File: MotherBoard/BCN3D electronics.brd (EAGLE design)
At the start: 80 x 140 mm, 139 parts, among them IC2 FT232RL, IC3 LMV324MZ, K1 G5L, Q1 MOSFET-N, Q2 MOSFET-N, Q3 MOSFET-N, Q4 BC817, Q5 BC817, Q9 BC817, X0 FFC_15V_90G_1MM, X1 FFC_15V_90G_1MM, Y0 FFC_15V_90G_1MM

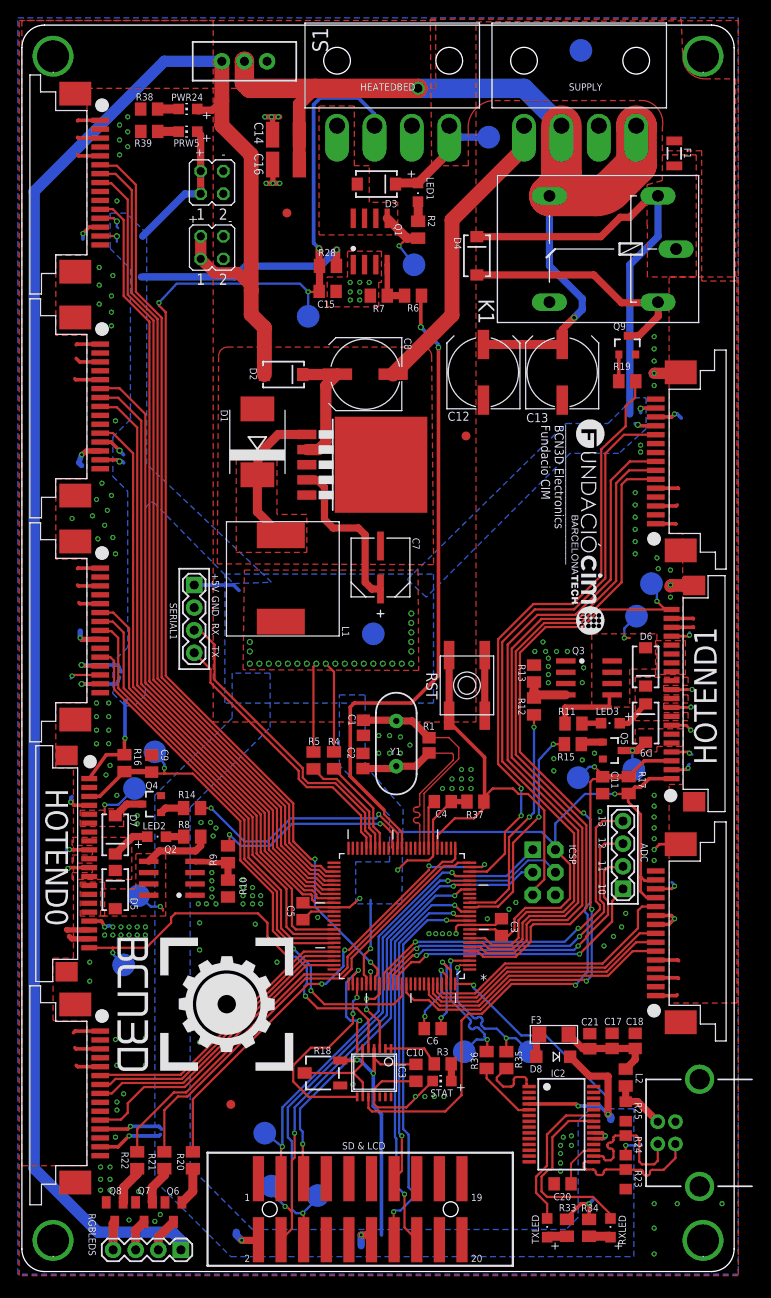
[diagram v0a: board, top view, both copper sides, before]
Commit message: BCN3D Electronics REV.E tested and manufactured
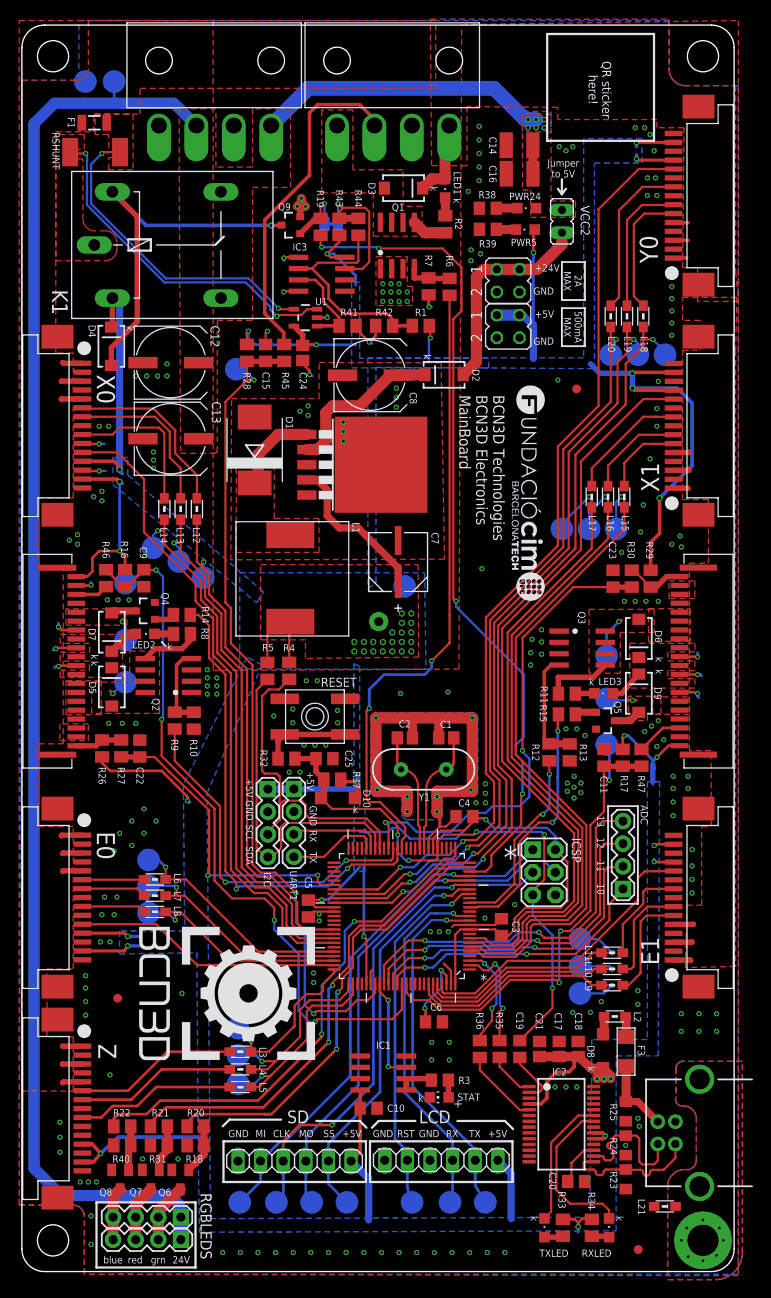
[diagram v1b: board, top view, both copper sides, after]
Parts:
- removed HTST1: HTST_20V_SMD_POL, MarcEagleParts:HTST-110-01-XX-DV
- removed JP1: +5V, jumper:JP2Q
- removed JP2: +24V, jumper:JP2Q
- removed PRW5: Red, adafruit:CHIP-LED0805
- removed RST: SPST_TACT-EVQQ2, adafruit:EVQ-Q2
- removed S1: (no value), SparkFun-Electromechanical:SWITCH-SPDT
- removed SERIAL1: (no value), SparkFun-Connectors:1X04
- removed TP14, TP18, TP6: TPB2,54, testpad:B2,54
- removed U$2, U$3, U$4: SANGUINOLOLU_PLATED-SCREW, SAV MK-I:SANGUINOLOLU_PLATEDSCREW
- added +24V, +5V: (no value), jumper:JP2Q
- added C19: 100n, rcl:C0805
- added C22, C23: 0.1u, rcl:C0805
- added C24: 100n, adafruit:C0805
- added C25: 10n, rcl:C0805
- added D10: MBR0520LT, diode:SOD123
- added I2C, LEDS1, UART1: (no value), SparkFun-Connectors:1X04
- added IC1: LM358D, linear:SO08
- added L10, L11, L12, L13, L14, L15, L16, L17, L18, L19, L20, L21, L3, L4, L5, L6, L7, L8, L9: (no value), EagleLibrary_Wuerth_Elektronik_eiSos_V6_20140807:0805
- added LCD, SD: (no value), pinhead:1X06
- added PWR5: Blue, led:CHIPLED_0805
- added R26, R29: 4.7K, rcl:M0805
- added R27, R30, R43, R45, R46, R47: 1K, rcl:M0805
- added R31, R40, R42: 10K, rcl:M0805
- added R32: 330, adafruit:M0805
- added R41: 20K, rcl:M0805
- added R44: 100K, rcl:M0805
- added RESET: SPST, adafruit:EVQ-Q2
- added RSHUNT: 10m, SparkFun-Resistors:R2512
- added SH1: SHORTT5, shorts:SHORT_TOP-50
- added SJ1: (no value), jumper:SJ
- added TP19, TP20, TP21, TP22, TP23, TP24, TP25, TP26, TP27, TP28, TP29, TP30, TP31, TP32, TP33, TP34, TP35, TP36, TP37, TP38: TPB2,54, testpad:B2,54
- added U1: INA169, SparkFun-AnalogIC:SOT23-5
- added VCC2: (no value), jumper:JP1
- C11, C15, C9: value 0.1u -> 10u
- HOTEND0, HOTEND1: value FFC_20V_90G_1MM" -> FFC_20V_90G_1MM3; device MarcEagleParts:SAMTEC_ZF1-T-WT -> MarcEagleParts:FCI_20WAY_1MM_3ST
- IC3: value LMV324MZ -> LM311D; device linear:TSSOP14 -> linear:SO08
- ICSP: value (none) -> AVR_SPI_PRG_6NS
- L2: value 1800367 Ferrite Bead -> (none); device rcl:M0805 -> EagleLibrary_Wuerth_Elektronik_eiSos_V6_20140807:0805
- LED1, LED2, LED3: value (none) -> Blue
- LM2595: device linear:TO263-5 -> MarcEagleParts:TO263-5
- PWR24: value Red -> Blue; device adafruit:CHIP-LED0805 -> led:CHIPLED_0805
- Q1, Q2, Q3: value MOSFET-N -> MOSFET-NSOIC8
- Q4, Q5, Q9: value BC817 -> MMBT2222A
- R1: value 1M -> 10K; device resistor:R0805 -> rcl:M0805
- R18: device pot:3223J -> rcl:M0805
- R4, R5: value 10K -> 4.7k
- U$1: value SANGUINOLOLU_PLATED-SCREW -> (none); device SAV MK-I:SANGUINOLOLU_PLATEDSCREW -> MarcEagleParts:BCN3D_QR
- moved Z 114.0 mm to (4.00, 18.3)
- moved U$1 112.6 mm to (60.4, 100.7), flipped to the bottom, turned to 270 degrees
- moved FID1 93.4 mm to (69.2, 2.48)
- moved IC3 89.9 mm to (33.7, 112.0), turned to 270 degrees
- moved TP13 83.4 mm to (24.1, 101.3), turned to 0 degrees
- moved TP5 73.1 mm to (48.1, 7.77), turned to 90 degrees
- moved Y0 71.3 mm to (76.0, 120.8), turned to 90 degrees
- moved F1 65.2 mm to (8.13, 129.0), turned to 180 degrees
- moved TP1 55.8 mm to (7.12, 133.7), turned to 0 degrees
- moved SUPPLY 47.2 mm to (21.9, 132.4)
- moved R1 47.1 mm to (44.8, 106.2), turned to 180 degrees
- moved K1 46.3 mm to (17.7, 115.3), turned to 0 degrees
- moved C13 44.6 mm to (16.7, 93.5), turned to 0 degrees
- moved TP2 42.5 mm to (10.4, 133.7), turned to 0 degrees
- moved D4 42.3 mm to (10.1, 103.9)
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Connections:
- removed net ATLVL0: HOTEND0.20, IC3.5, TP4.TP
- removed net ATLVL1: HOTEND1.20, IC3.10, TP5.TP
- removed net H0-STOP: ATMEGA2560.77, IC3.7
- removed net H1-STOP: ATMEGA2560.78, IC3.8
- removed net N$108: C12.+, C13.+, C14.1, C16.1, K1.S, S1.2, SUPPLY.1, SUPPLY.3
- removed net N$110: IC3.6, IC3.9, R18.2
- removed net N$111: HTST1.8
- removed net N$112: HTST1.9
- removed net N$115: HTST1.10
- removed net N$116: HTST1.16
- removed net N$117: HTST1.17
- removed net N$118: HTST1.18
- removed net N$119: HTST1.19
- removed net N$120: HTST1.20
- removed net N$121: S1.1
- removed net N$124: ATMEGA2560.18
- removed net N$146: ATMEGA2560.41
- removed net N$25: Q9.1, R19.1
- removed net RX0: ATMEGA2560.2, R35.1, TP13.TP
- removed net TX0: ATMEGA2560.3, R36.1, TP14.TP
- removed net VBUSAF: C17.1, C18.1, C21.1, F3.2, L2.1
- new net 24VINA: K1.P, RSHUNT.1, U1.3
- new net BED_THERM_CON: HEATEDBED.3, R45.1
- new net EARTH: L21.2, U$6.S1, U$6.S2
- new net GUARD: C1.2, C2.2, SH1.2
- new net HOTEND0_THERM_CON: HOTEND0.3, R46.1
- new net HOTEND1_THERM_CON: HOTEND1.3, R47.1
- new net INA_OUT: IC3.3, R41.2, U1.1
- new net N$1: C19.1, IC2.2
- new net N$34: L13.1, X0.7
- new net N$35: L14.1, X0.9
- new net N$36: L18.1, Y0.6
- new net N$37: L19.1, Y0.7
- new net N$39: L20.1, Y0.9
- new net N$4: ATMEGA2560.14
- new net N$40: L15.1, X1.6
- new net N$41: L16.1, X1.7
- new net N$42: L17.1, X1.9
- new net N$43: E0.6, L6.2
- new net N$44: E0.7, L7.2
- new net N$45: E0.9, L8.2
- new net N$47: ATMEGA2560.55
- new net N$48: F3.2, L2.1
- new net N$49: IC3.2, R1.2, R42.1, R44.1
- new net N$5: L12.1, X0.6
- new net N$54: L3.1, Z.6
- new net N$55: L4.1, Z.7
- new net N$56: L5.1, Z.9
- new net N$57: E1.9, L11.1
- new net N$58: E1.7, L10.1
- new net N$59: E1.6, L9.1
- new net RELAYINA: IC3.7, Q9.1, R19.1, R43.2, R44.2, SJ1.1, SJ1.2
- new net SUPPLY: C12.+, C13.+, C14.1, C16.1, K1.S, LEDS1.1, PWR24.A, RGBLEDS.1, SUPPLY.1, SUPPLY.3, TP2.TP, VCC2.1
- new net UART_N: ATMEGA2560.3, R36.1
- new net UART_P: ATMEGA2560.2, R35.1
- new net Z0-ENDSTOP: HOTEND0.20, R26.1, R27.1
- new net Z0-STOP: ATMEGA2560.56, C22.1, R27.2
- new net Z1-ENDSTOP: HOTEND1.20, R29.1, R30.1
- new net Z1-STOP: ATMEGA2560.41, C23.1, R30.2
- net !RESET: now also C19.2, C25.1, D10.A, R32.1; no longer RST.A, RST.A'
- net +24V: now also Y0.GND@2; no longer HOTEND1.GND1, TP2.TP, Z.GND@1
- net +5V: now also +24V.1, +24V.3, C17.1, C18.1, C21.1, C24.1, D10.C, I2C.1, IC1.8, IC3.8, LCD.1, PWR5.A, R1.1, R26.2, R29.2, R43.1, SD.6, U1.5, UART1.1; no longer HTST1.1, HTST1.11, IC3.4, JP1.1, JP1.3, PRW5.A, R18.3, SERIAL1.1
- net 24VBF: now also RSHUNT.2, U1.4; no longer K1.P
- net BED_THERM: now also R45.2, TP13.TP; no longer HEATEDBED.3, TP18.TP
- net E0-!EN: now also L7.1, TP34.TP; no longer E0.7
- net E0-DIR: now also ATMEGA2560.73, L8.1, TP33.TP; no longer ATMEGA2560.71, E0.6
- net E0-STEP: now also ATMEGA2560.71, L6.1, TP35.TP; no longer ATMEGA2560.73, E0.8
- net E1-!EN: now also L10.2, TP31.TP; no longer E1.7
- net E1-DIR: now also ATMEGA2560.96, L11.2, TP32.TP; no longer ATMEGA2560.94, E1.6
- net E1-STEP: now also ATMEGA2560.94, L9.2, TP30.TP; no longer ATMEGA2560.96, E1.8
- net GND: now also +24V.2, +24V.4, +5V.2, +5V.4, C22.2, C23.2, C24.2, C25.2, E0.8, E1.8, HOTEND1.GND1, I2C.2, IC1.4, IC3.1, IC3.4, L21.1, LCD.4, LCD.6, R18.2, R31.2, R40.2, R41.1, R42.2, RESET.A, RESET.A', SD.1, SH1.1, U1.2, UART1.2, X0.8, X1.8, Y0.8, Z.8, Z.GND@1; no longer C1.2, C2.2, E0.9, E1.9, HTST1.12, HTST1.2, IC3.11, JP1.2, JP1.4, JP2.2, JP2.4, R18.1, RST.B, RST.B', SERIAL1.2, U$1.GND, U$2.GND, U$3.GND, U$4.GND, U$6.S1, U$6.S2, X0.9, X1.9, Y0.9, Y0.GND@2, Z.9
- net HOTBED: no longer TP6.TP
- net HOTEND0_THERM: now also R46.2; no longer HOTEND0.3
- net HOTEND1_THERM: now also R47.2; no longer HOTEND1.3
- net LCDRESET: now also ATMEGA2560.18, LCD.5, TP4.TP; no longer ATMEGA2560.14, HTST1.15
- net LCDRX: now also LCD.3, TP5.TP; no longer HTST1.14
- net LCDTX: now also LCD.2, TP15.TP; no longer HTST1.13
- net MISO: now also SD.2, TP20.TP; no longer HTST1.4, TP16.TP
- net MLED: now also IC1.3; no longer IC3.3
- net MOSI: now also SD.4, TP17.TP; no longer HTST1.5, TP15.TP
- net N$10: now also LEDS1.3
- net N$11: now also LEDS1.4
- net N$13: now also R32.2, RESET.B, RESET.B'; no longer IC2.2
- net N$162: now also PWR5.C; no longer PRW5.C
- net N$23: now also L2.2; no longer F3.1
- net N$24: now also ATMEGA2560.78; no longer HTST1.7
- net N$26: now also IC1.1, IC1.2; no longer IC3.1, IC3.2
- net N$27: now also R18.1
- net N$29: now also ATMEGA2560.53; no longer ATMEGA2560.76
- net N$31: now also R31.1
- net N$32: now also R40.1
- net N$33: now also ATMEGA2560.54; no longer ATMEGA2560.75
- net N$9: now also LEDS1.2
- net RX1: now also UART1.3; no longer SERIAL1.3
- net SCL: now also I2C.3
- net SCLK: now also SD.3, TP19.TP; no longer HTST1.3, TP17.TP
- net SDA: now also I2C.4
- net SDSS: now also SD.5, TP16.TP; no longer HTST1.6
- net TX1: now also UART1.4; no longer SERIAL1.4
- net VBUS: now also F3.1; no longer L2.2
- net VCC2: now also +5V.1, +5V.3, VCC2.2; no longer JP2.1, JP2.3, PWR24.A, RGBLEDS.1, S1.3
- net X0-!EN: now also L13.2, TP22.TP; no longer X0.7
- net X0-DIR: now also ATMEGA2560.68, L14.2, TP23.TP; no longer ATMEGA2560.66, X0.6
- net X0-STEP: now also ATMEGA2560.66, L12.2, TP21.TP; no longer ATMEGA2560.68, X0.8
- net X1-!EN: now also L16.2, TP25.TP; no longer X1.7
- net X1-DIR: now also ATMEGA2560.7, L17.2, TP26.TP; no longer ATMEGA2560.5, X1.6
- net X1-STEP: now also ATMEGA2560.5, L15.2, TP24.TP; no longer ATMEGA2560.7, X1.8
- net XTAL_N: no longer R1.2
- net XTAL_P: no longer R1.1
- net Y-!EN: now also ATMEGA2560.59, L19.2, TP28.TP; no longer ATMEGA2560.58, Y0.7
- net Y-DIR: now also ATMEGA2560.58, L20.2, TP29.TP; no longer ATMEGA2560.57, Y0.6
- net Y-STEP: now also ATMEGA2560.60, L18.2, TP27.TP; no longer ATMEGA2560.59, Y0.8
- net Y-STOP: now also ATMEGA2560.57; no longer ATMEGA2560.60
- net Z-!EN: now also ATMEGA2560.76, L4.2, TP37.TP; no longer ATMEGA2560.54, Z.7
- net Z-DIR: now also ATMEGA2560.77, L5.2, TP36.TP; no longer ATMEGA2560.53, Z.6
- net Z-STEP: now also ATMEGA2560.75, L3.2, TP38.TP; no longer ATMEGA2560.55, Z.8
- net Z-STOP: no longer ATMEGA2560.56
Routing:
- net SUPPLY: track 0.00 -> 198.5 mm, vias 0 -> 6
- net VCC2: track 208.3 -> 24.1 mm
- net N$108: track 101.0 -> 0.00 mm, vias 2 -> 0
- net ATLVL1: track 100.7 -> 0.00 mm, vias 3 -> 0
- net Z-STOP: track 88.9 -> 0.00 mm
- net GND: track 151.9 -> 64.2 mm, vias 215 -> 234
- net Z-STEP: track 91.1 -> 18.8 mm, vias 0 -> 1
- net Z-!EN: track 91.9 -> 22.0 mm, vias 0 -> 1
- net Z-DIR: track 92.4 -> 22.8 mm, vias 0 -> 1
- net Z1-STOP: track 0.00 -> 54.1 mm, vias 0 -> 2
- net ATLVL0: track 47.0 -> 0.00 mm, vias 3 -> 0
- net GUARD: track 0.00 -> 45.0 mm, vias 0 -> 8
- net BED_THERM: track 139.6 -> 95.7 mm, vias 5 -> 3
- net Y-STOP: track 66.2 -> 105.9 mm, vias 0 -> 2
- net 24VINA: track 0.00 -> 39.3 mm, vias 0 -> 2
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- added copper zone on layer 1, net 24VINA
- added copper zone on layer 1, net EARTH
- added copper zone on layer 16, net EARTH
- added copper zone on layer 16, net GUARD
- added copper zone on layer 1, net SUPPLY
- added copper zone on layer 16, net SUPPLY
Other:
- board text added: "*"
- board text added: "+24V"
- board text added: "24V"
- board text added: "2A MAX"
- board text added: "500mA MAX"
- board text added: "BCN3D Technologies BCN3D Electronics MainBoard"
- board text added: "BCN3D Technologies BCN3D Electronics MainBoard v1.0 Designed in Barcelona ___________________ Sep 2015 - REV_E"
- board text added: "CLK"
- board text added: "E0"
- board text added: "E1"
- board text added: "For more info scan QR Code"
- board text added: "HB"
- board text added: "Jumper to 5V"
- board text added: "MI"
- board text added: "MO"
- board text added: "QR sticker here!"
- board text added: "RST"
- board text added: "SCL"
- board text added: "SDA"
- board text added: "SS"
- board text added: "THERM"
- board text added: "X0"
- board text added: "X1"
- board text added: "Y0"
- board text added: "Z"
- board text added: "blue"
- board text added: "grn"
- board text added: "k"
- board text added: "red"
- board text removed: "+"
- board text removed: "-"
- board text removed: "1"
- board text removed: "19"
- board text removed: "2"
- board text removed: "20"
- board text removed: "BCN3D Electronics MainBoard v1.0 Designed in Barcelona ___________________ MotherBoard - Jan 2015 Marc Cobler - REV_B ___________________"
- board text removed: "SD & LCD"
- board text removed: "_________________________ BCN3D Electronics Fundacio CIM"
